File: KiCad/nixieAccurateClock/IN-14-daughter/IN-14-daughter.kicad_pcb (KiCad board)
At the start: 4 copper layers, 19 x 32 mm, 12 parts, among them J1 Conn_02x05_Odd_Even, U1 HV509K6-G

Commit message: switch to 27k R_anode
Add voltage rail jumpers for different 5V and 3.3V standby applications
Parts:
- R1: value 33k -> 27k
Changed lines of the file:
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@@
     (descr "Resistor SMD 1206 (3216 Metric), square (rectangular) end terminal, IPC_7351 nominal, (Body size source: IPC-SM-782 page 72, https://www.pcb-3d.com/wordpress/wp-content/uploads/ipc-sm-782a_amendment_1_and_2.pdf), generated with kicad-footprint-generator")
     (tags "resistor")
-    (property "Digikey link" "https://www.digikey.com/en/products/detail/yageo/RC1206JR-0733KL/729282")
-    (property "Model" "RC1206JR-0733KL")
-    (property "Mouser link" "https://www.mouser.com/ProductDetail/YAGEO/RC1206JR-0733KL?qs=4sq2y2bXwtTBbhYRyjZ6aQ%3D%3D")
+    (property "Digikey link" "https://www.digikey.com/en/products/detail/yageo/RC1206JR-0727KL/729262")
+    (property "Model" "RC1206JR-0727KL")
+    (property "Mouser link" "https://www.mouser.com/ProductDetail/YAGEO/RC1206JR-0727KL?qs=CteSnpDdeuBg3%2FC0aG6GFQ%3D%3D")
     (property "Price" "0.10")
     (property "Sheetfile" "IN-14-daughter.kicad_sch")
@@
         (effects (font (size 1 1) (thickness 0.15)) (justify mirror))
     )
-    (fp_text value "33k" (at 0 -1.82) (layer "B.Fab")
+    (fp_text value "27k" (at 0 -1.82) (layer "B.Fab")
         (effects (font (size 1 1) (thickness 0.15)) (justify mirror))
     )

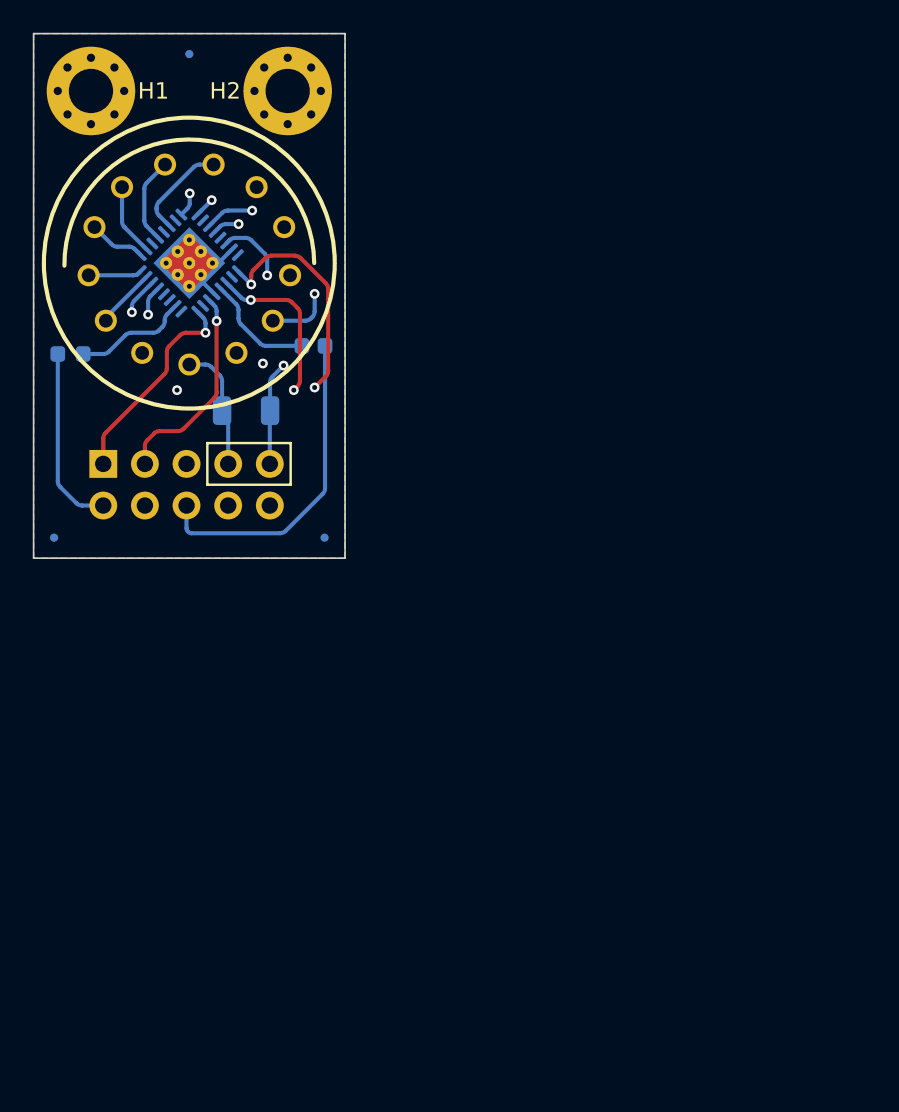
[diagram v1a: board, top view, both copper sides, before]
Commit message: add board info to drawings
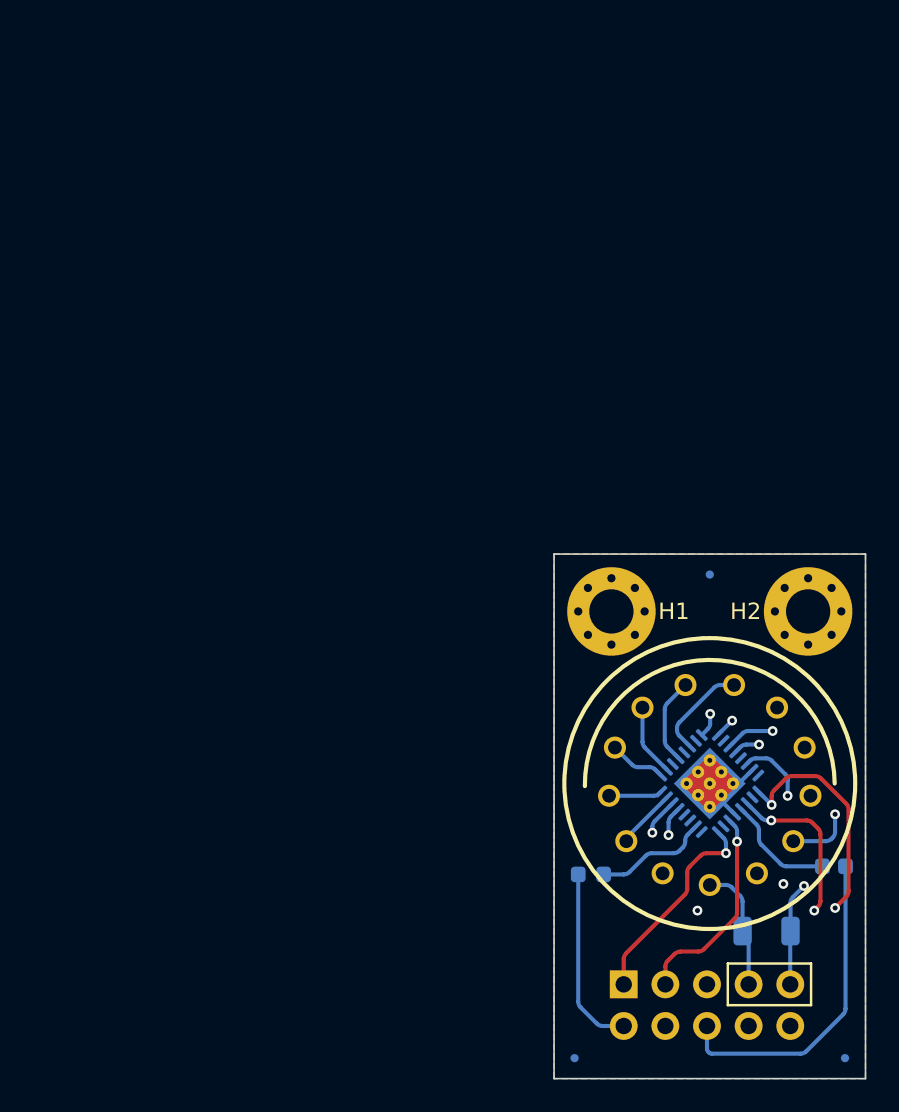
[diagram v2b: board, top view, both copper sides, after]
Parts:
- moved C1 44.9 mm to (48.9, 50.8)
- moved C2 44.9 mm to (34.0, 51.3)
- moved FID1 44.9 mm to (33.0, 62.5)
- moved FID2 44.9 mm to (49.5, 62.5)
- moved FID3 44.9 mm to (41.2, 33.0)
- moved H1 44.9 mm to (35.2, 35.2)
- moved H2 44.9 mm to (47.2, 35.2)
- moved J1 44.9 mm to (36.0, 58.0)
- moved N1 44.9 mm to (41.2, 45.8)
- moved R1 44.9 mm to (44.7, 54.8)
- moved REF** 44.9 mm to (48.2, 57.7)
- moved U1 44.9 mm to (41.2, 45.8)
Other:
- board text added: "0"
- board text added: "0 mm"
- board text added: "0.0000 mm / 0.0000 mm"
- board text added: "0.01 mm"
- board text added: "0.02"
- board text added: "0.0525 mm"
- board text added: "0.07 mm"
- board text added: "0.22 mm"
- board text added: "0.3000 mm"
- board text added: "0.895 mm"
- board text added: "1"
- board text added: "1.6000 mm"
- board text added: "19.0000 mm x 32.0000 mm"
- board text added: "3.3"
- board text added: "4"
- board text added: "4.5"
- board text added: "B.Cu"
- board text added: "B.Mask"
- board text added: "B.Paste"
- board text added: "B.Silkscreen"
- board text added: "BOARD CHARACTERISTICS"
- board text added: "Black"
- board text added: "Board Thickness:"
- board text added: "Board overall dimensions:"
- board text added: "Bottom Silk Screen"
- board text added: "Bottom Solder Mask"
- board text added: "Bottom Solder Paste"
- board text added: "Castellated pads:"
- board text added: "Color"
- board text added: "Copper Finish:"
- board text added: "Copper Layer Count:"
- board text added: "Dielectric 1"
- board text added: "Dielectric 2"
- board text added: "Dielectric 3"
- board text added: "ENIG"
- board text added: "Edge card connectors:"
- board text added: "Epsilon R"
- board text added: "F.Cu"
- board text added: "F.Mask"
- board text added: "F.Paste"
- board text added: "F.Silkscreen"
- board text added: "FR4"
- board text added: "FR4 natural"
- board text added: "Impedance Control:"
- board text added: "In1.Cu"
- board text added: "In2.Cu"
- board text added: "Layer Name"
- board text added: "Loss Tangent"
- board text added: "Material"
- board text added: "Min hole diameter:"
- board text added: "Min track/spacing:"
- board text added: "No"
- board text added: "Not specified"
- board text added: "Plated Board Edge:"
- board text added: "Thickness (mm)"
- board text added: "Top Silk Screen"
- board text added: "Top Solder Mask"
- board text added: "Top Solder Paste"
- board text added: "Type"
- board text added: "White"
- board text added: "copper"
- board text added: "core"
- board text added: "prepreg"

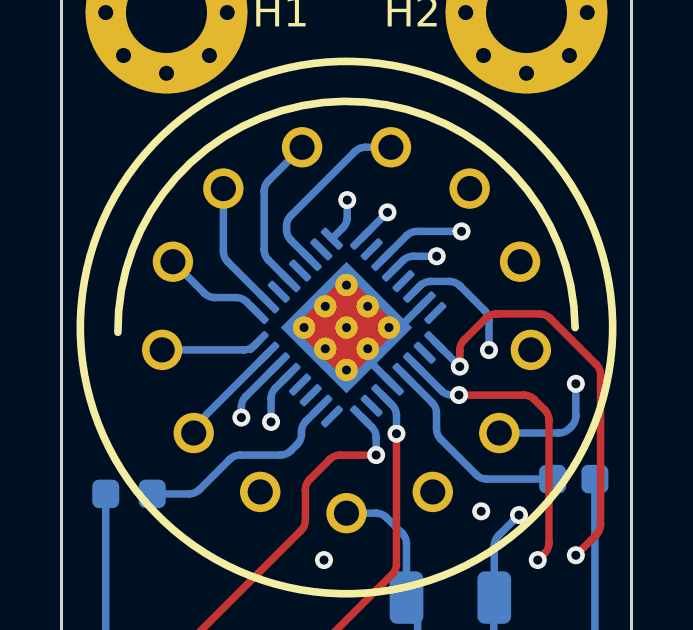
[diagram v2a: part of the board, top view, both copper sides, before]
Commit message: configure outjobs
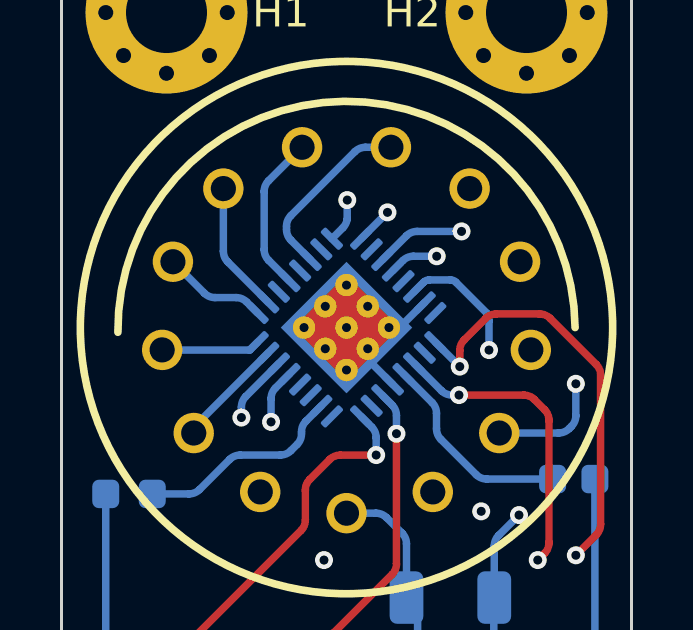
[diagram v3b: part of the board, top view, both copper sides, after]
